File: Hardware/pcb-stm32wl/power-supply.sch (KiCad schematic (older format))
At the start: 45 parts, among them Q1 SI2323DS, U1 TPS22917DBV, U2 RP605Z283B, U3 TPS22917DBV, U4 TPS22917DBV

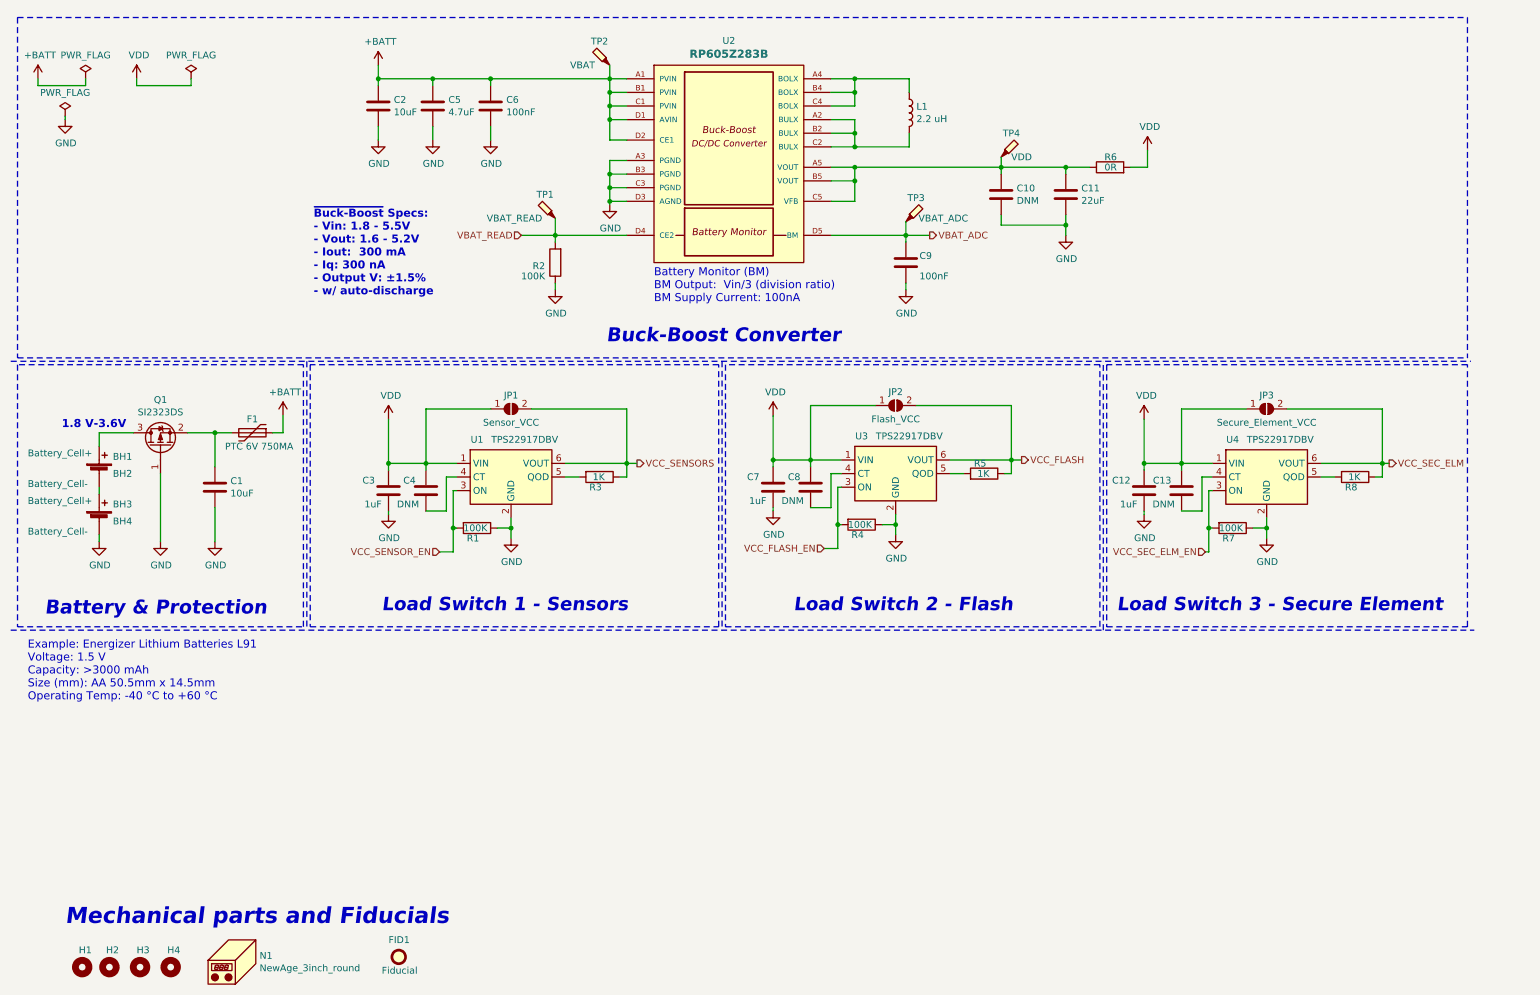
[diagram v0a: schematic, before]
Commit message: hw: Update latest design files and Readme
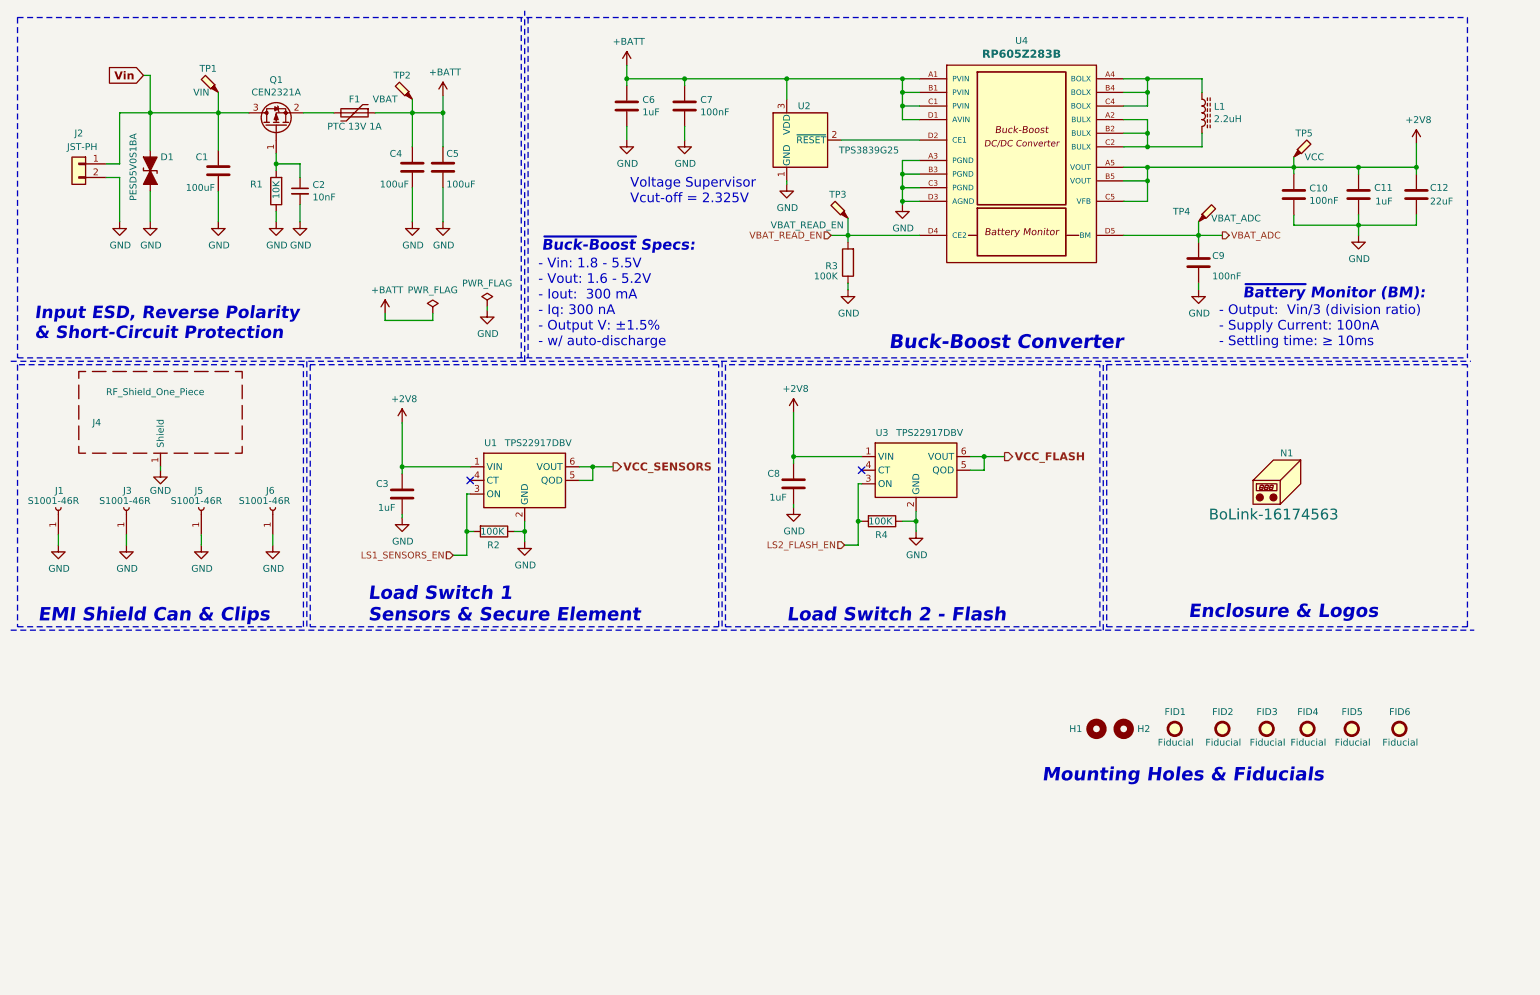
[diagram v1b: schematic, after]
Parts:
- removed BH1, BH3: Battery_Cell+, node-lib-v1:BAT_BK-92, symbol node-lib-v1:Battery_Cell+
- removed BH2, BH4: Battery_Cell-, node-lib-v1:BAT_BK-92, symbol node-lib-v1:Battery_Cell-
- removed C12: 1uF, Capacitor_SMD:C_0402_1005Metric, symbol Device:C
- removed C13, C8: DNM, Capacitor_SMD:C_0402_1005Metric, symbol Device:C
- removed C2: 10uF, Capacitor_SMD:C_0603_1608Metric, symbol Device:C
- removed H3, H4: MountingHole, MountingHole:MountingHole_2.5mm, symbol Mechanical:MountingHole
- removed JP1: Sensor_VCC, Jumper:SolderJumper-2_P1.3mm_Open_RoundedPad1.0x1.5mm, symbol Jumper:SolderJumper_2_Open
- removed JP2: Flash_VCC, Jumper:SolderJumper-2_P1.3mm_Open_RoundedPad1.0x1.5mm, symbol Jumper:SolderJumper_2_Open
- removed JP3: Secure_Element_VCC, Jumper:SolderJumper-2_P1.3mm_Open_RoundedPad1.0x1.5mm, symbol Jumper:SolderJumper_2_Open
- removed L1: 2.2 uH, Inductor_SMD:L_1008_2520Metric, symbol Device:L
- removed R3, R5, R8: 1K, Resistor_SMD:R_0402_1005Metric, symbol Device:R
- removed R6: 0R, Resistor_SMD:R_0402_1005Metric, symbol Device:R
- removed R7: 100K, Resistor_SMD:R_0402_1005Metric, symbol Device:R
- removed U4: TPS22917DBV, Package_TO_SOT_SMD:SOT-23-6, symbol Power_Management:TPS22917DBV
- added C11: 1uF, Capacitor_SMD:C_0402_1005Metric, symbol Device:C
- added C2: 10nF, Capacitor_SMD:C_0402_1005Metric, symbol Device:C_Small
- added C5: 100uF, Capacitor_SMD:C_1206_3216Metric, symbol Device:C
- added D1: PESD5V0S1BA, Diode_SMD:D_SOD-323, symbol Device:D_TVS_ALT
- added FID2, FID3, FID4, FID5, FID6: Fiducial, Fiducial:Fiducial_0.5mm_Mask1.5mm, symbol Mechanical:Fiducial
- added J1, J3, J5, J6: S1001-46R, node-lib-v1:RF_Shield_Clip_S1001-46R, symbol Connector:Conn_01x01_Female
- added J2: JST-PH, Connector_JST:JST_PH_B2B-PH-SM4-TB_1x02-1MP_P2.00mm_Vertical, symbol Connector_Generic:Conn_01x02
- added J4: RF_Shield_One_Piece, node-lib-v1:RF_Shield_SnapOn_30x20mm_w_Cutout_n_GND_Pads, symbol Device:RF_Shield_One_Piece
- added L1: 2.2uH, node-lib-v1:L_HPC4012TF-2R2M, symbol Device:L_Core_Ferrite
- added R1: 10K, Resistor_SMD:R_0402_1005Metric, symbol Device:R
- added TP1: VIN, TestPoint:TestPoint_Pad_D1.5mm, symbol Connector:TestPoint_Probe
- added U2: TPS3839G25, Package_TO_SOT_SMD:SOT-23, symbol Power_Supervisor:TPS3839DBZ
- C1: value 10uF -> 100uF; footprint Capacitor_SMD:C_0603_1608Metric -> Capacitor_SMD:C_1206_3216Metric; MPN C1608X5R0J106K080AB -> JMK316ABJ107ML-T; URL (none) -> https://lcsc.com/product-detail/Multilayer-Ceramic-Capacito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
- C10: value DNM -> 100nF; footprint Capacitor_SMD:C_0603_1608Metric -> Capacitor_SMD:C_0402_1005Metric; MPN (none) -> CC0402KRX7R7BB104; URL (none) -> https://lcsc.com/product-detail/Multilayer-Ceramic-Capacito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
- C12: renamed from C11; ALT_MPN (none) -> JMK107BBJ226MA; MPN JMK107BBJ226MA -> CC0603MRX5R5BB226; URL (none) -> https://lcsc.com/product-detail/Multilayer-Ceramic-Capacito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
- C3, C9: URL (none) -> https://lcsc.com/product-detail/Multilayer-Ceramic-Capacito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
- C4: value DNM -> 100uF; footprint Capacitor_SMD:C_0402_1005Metric -> Capacitor_SMD:C_1206_3216Metric; MPN (none) -> JMK316ABJ107ML-T; URL (none) -> https://lcsc.com/product-detail/Multilayer-Ceramic-Capacito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
- C6: renamed from C5; value 4.7uF -> 1uF; footprint Capacitor_SMD:C_0603_1608Metric -> Capacitor_SMD:C_0402_1005Metric; MPN C1608X5R1C475K080AC -> CL05A105KQ5NNNC; URL (none) -> https://lcsc.com/product-detail/Multilayer-Ceramic-Capacito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
- C7: renamed from C6; URL (none) -> https://lcsc.com/product-detail/Multilayer-Ceramic-Capacito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
- C8: renamed from C7; URL (none) -> https://lcsc.com/product-detail/Multilayer-Ceramic-Capacito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
- F1: value PTC 6V 750MA -> PTC 13V 1A; footprint node-lib-v1:Fuse_0805_2012Metric_Castellated -> Fuse:Fuse_1210_3225Metric_Castellated; MPN 0ZCK0075FF2E -> SMD1210-050; URL (none) -> https://lcsc.com/product-detail/PTC-Resettable-Fuses_TECHFU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
- N1: value NewAge_3inch_round -> BoLink-16174563; footprint node-lib-v1:NewAge_3inch_round -> node-lib-v1:BoLink_704025; ALT_MPN (none) -> S6L-303013; MPN S6L-303013 -> DNM; URL (none) -> https://www.distrelec.nl/en/bolink-iot-enclosure-bolink-43-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
- Q1: value SI2323DS -> CEN2321A; MPN SI2323DS-T1-E3 -> CEN2321A; URL (none) -> https://lcsc.com/product-detail/MOSFET_CET-Chino-Excel-Tech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
- R2: renamed from R1; URL (none) -> https://lcsc.com/product-detail/Chip-Resistor-Surface-Mount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
- R3: renamed from R2; URL (none) -> https://lcsc.com/product-detail/Chip-Resistor-Surface-Mount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
- R4: URL (none) -> https://lcsc.com/product-detail/Chip-Resistor-Surface-Mount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
- TP2: footprint TestPoint:TestPoint_Pad_D1.0mm -> TestPoint:TestPoint_Pad_D1.5mm; MPN (none) -> DNM
- TP3: renamed from TP1; value VBAT_READ -> VBAT_READ_EN; footprint TestPoint:TestPoint_Pad_D1.0mm -> TestPoint:TestPoint_Pad_D1.5mm; MPN (none) -> DNM
- TP4: renamed from TP3; footprint TestPoint:TestPoint_Pad_D1.0mm -> TestPoint:TestPoint_Pad_D1.5mm; MPN (none) -> DNM
- TP5: renamed from TP4; value VDD -> VCC; footprint TestPoint:TestPoint_Pad_D1.0mm -> TestPoint:TestPoint_Pad_D1.5mm; MPN (none) -> DNM
- U1, U3: URL (none) -> https://www.ti.com/store/ti/en/p/product/?p=TPS22917DBVR
- U4: renamed from U2; URL (none) -> https://eu.mouser.com/ProductDetail/Ricoh-Electronic-Device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
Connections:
- net +BATT: now also C4.2, C5.2, U2.3 (VDD); no longer U4.D2 (CE1)
- net GND: now also C4.1, C11.2, C2.2, C5.1, D1.2 (A2), J1.1 (Pin_1), J2.2 (Pin_2), J3.1 (Pin_1), J4.1 (Shield), J5.1 (Pin_1), J6.1 (Pin_1), R1.1, U2.1 (GND); no longer Q1.1 (G)
- net VCC_FLASH: now also U3.5 (QOD)
- net VCC_SENSORS: now also U1.5 (QOD)
- net at F1.2, Q1.2 (S): no longer C1.2
- net Vin: now reaches Q1.3 (D)
- net Vin: now also C1.2, D1.1 (A1), J2.1 (Pin_1), TP1.1
- net at U1.4 (CT): no longer C4.2
- net +2V8: now reaches C10.2, C12.2, TP5.1, U4.A5 (VOUT), U4.B5 (VOUT), U4.C5 (VFB)
- net +2V8: now also C3.1, C8.1, U1.1 (VIN), U3.1 (VIN), C11.1
- net at U4.A2 (BULX), U4.B2 (BULX), U4.C2 (BULX): now also L1.2
- net at U4.A4 (BOLX), U4.B4 (BOLX), U4.C4 (BOLX): now also L1.1
- net VBAT_READ renamed VBAT_READ_EN
- net VCC_FLASH_EN renamed LS2_FLASH_EN
- net VCC_SENSOR_EN renamed LS1_SENSORS_EN
- removed net VDD: C3.1, C4.1, C8.1, U1.1 (VIN), U3.1 (VIN)
- new net: C2.1, Q1.1 (G), R1.2
- new net: U2.2 (~RESET), U4.D2 (CE1)
- no-connect marks 0 -> 2
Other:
- note added: "- Output: Vin/3 (division ratio)\n- Supply Current: 100nA\n- Settling time: ≥ 10ms"
- note added: "- Vin: 1.8 - 5.5V\n- Vout: 1.6 - 5.2V\n- Iout: 300 mA\n- Iq: 300 nA\n- Output V: ±1.5%\n- w/ auto-discharge"
- note added: "EMI Shield Can & Clips"
- note added: "Enclosure & Logos"
- note added: "Input ESD, Reverse Polarity \n& Short-Circuit Protection"
- note added: "Load Switch 1 \nSensors & Secure Element"
- note added: "Mounting Holes & Fiducials"
- note added: "Voltage Supervisor\nVcut-off = 2.325V"
- note added: "~Battery Monitor (BM):"
- note added: "~Buck-Boost Specs:"
- note removed: "1.8 V-3.6V"
- note removed: "Battery & Protection"
- note removed: "Battery Monitor (BM)\nBM Output: Vin/3 (division ratio)\nBM Supply Current: 100nA"
- note removed: "Example: Energizer Lithium Batteries L91\nVoltage: 1.5 V\nCapacity: >3000 mAh\nSize (mm): AA 50.5mm x 14.5mm \nOperating Temp: -40 °C to +60 °C"
- note removed: "Load Switch 1 - Sensors"
- note removed: "Load Switch 3 - Secure Element"
- note removed: "Mechanical parts and Fiducials"
- note removed: "~Buck-Boost Specs:\n- Vin: 1.8 - 5.5V\n- Vout: 1.6 - 5.2V\n- Iout: 300 mA\n- Iq: 300 nA\n- Output V: ±1.5%\n- w/ auto-discharge"
- moved on the sheet: C10, C12, C3, C6, C7, C8, C9, F1, FID1, H1, H2, N1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
